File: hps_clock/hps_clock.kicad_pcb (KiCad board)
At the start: 2 copper layers, 118 x 118 mm, 4 parts

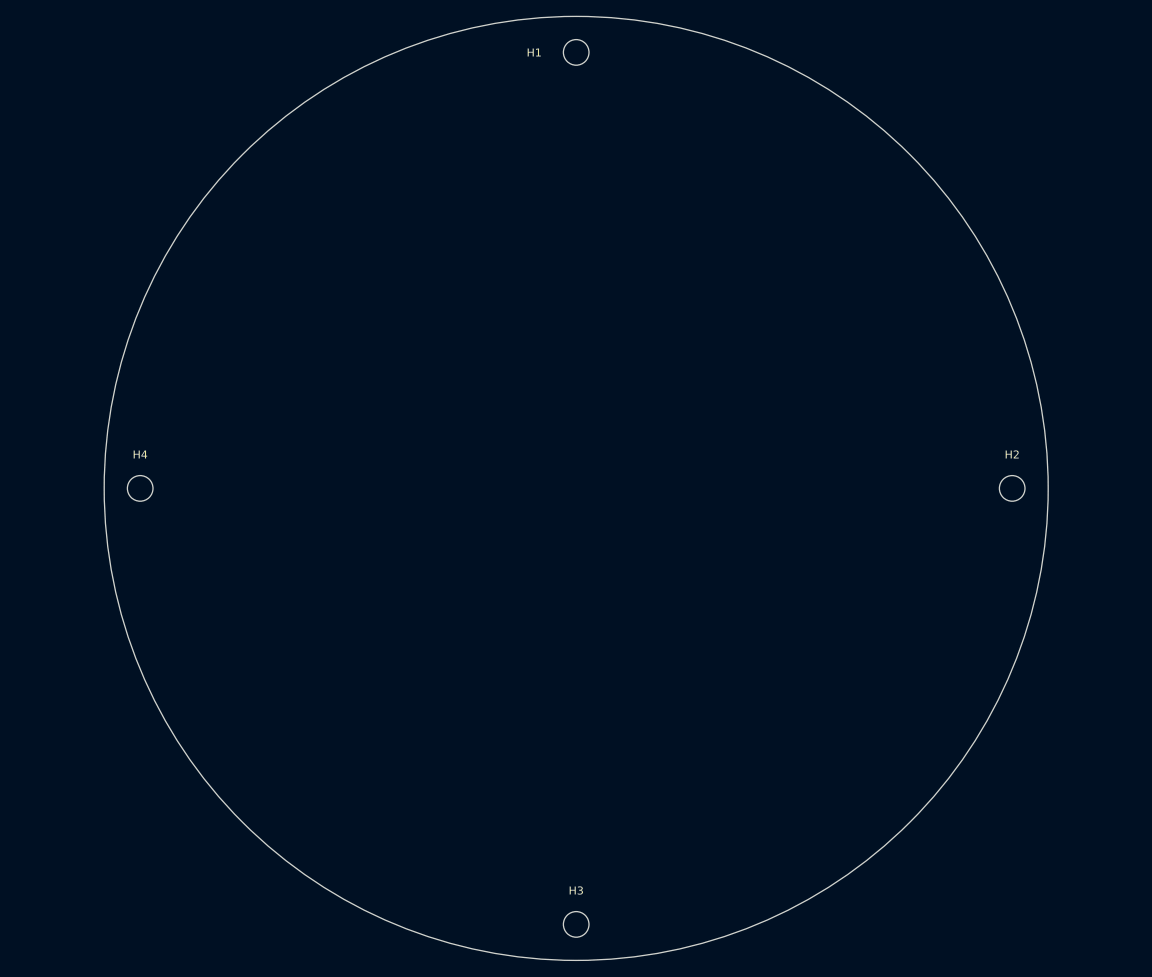
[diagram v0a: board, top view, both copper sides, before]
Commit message: schematic done..?
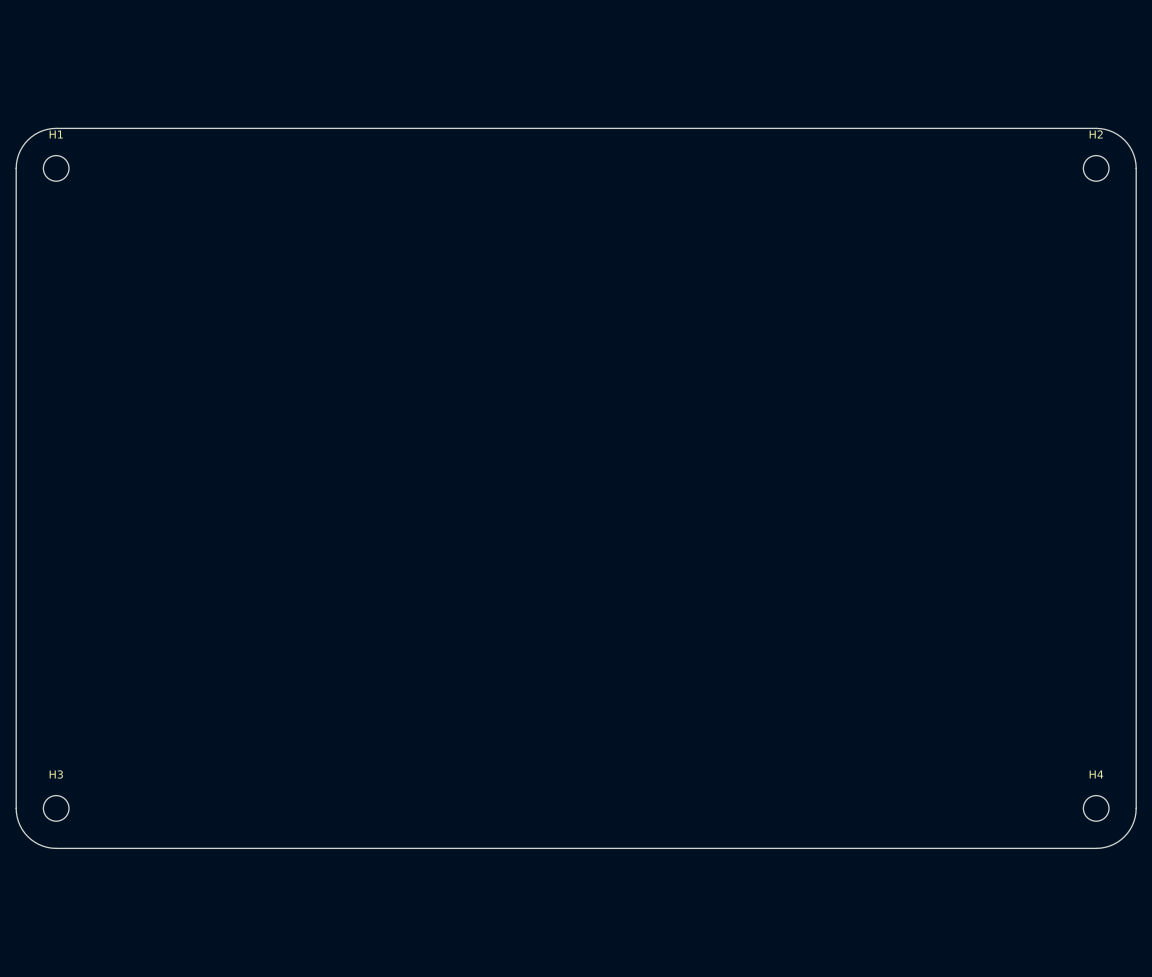
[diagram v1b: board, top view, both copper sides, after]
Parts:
- moved H4 126.0 mm to (215.0, 140.0)
- moved H1 66.6 mm to (85.0, 60.0)
- moved H3 66.6 mm to (85.0, 140.0)
- moved H2 41.4 mm to (215.0, 60.0)
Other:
- board size 118 x 118 mm -> 140 x 90 mm
